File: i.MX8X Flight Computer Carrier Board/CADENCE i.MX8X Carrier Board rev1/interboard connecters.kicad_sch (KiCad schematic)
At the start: 54 parts, among them CN2 DF11-16DP-2DSA(08), CN3 DF11-16DP-2DSA(08), CN4 DF11-16DP-2DSA(08), J10 Conn_01x04, J11 Conn_01x04, J13 Conn_01x04, J16 Conn_01x04, J17 Conn_01x04, J21 Conn_02x02_Odd_Even, J22 Conn_01x04, J23 Conn_01x04, J24 Conn_01x05, J25 Conn_01x05, J27 Conn_01x04, J6 Conn_01x01, J7 Conn_01x08, J8 Conn_02x26_Odd_Even, J9 Conn_02x26_Odd_Even, U33 SN65HVD233, U34 INA219AxDCN, U35 TPS22810DBV, U36 INA219AxDCN, U37 TPS22810DBV, U38 INA219AxDCN, U39 TPS22975

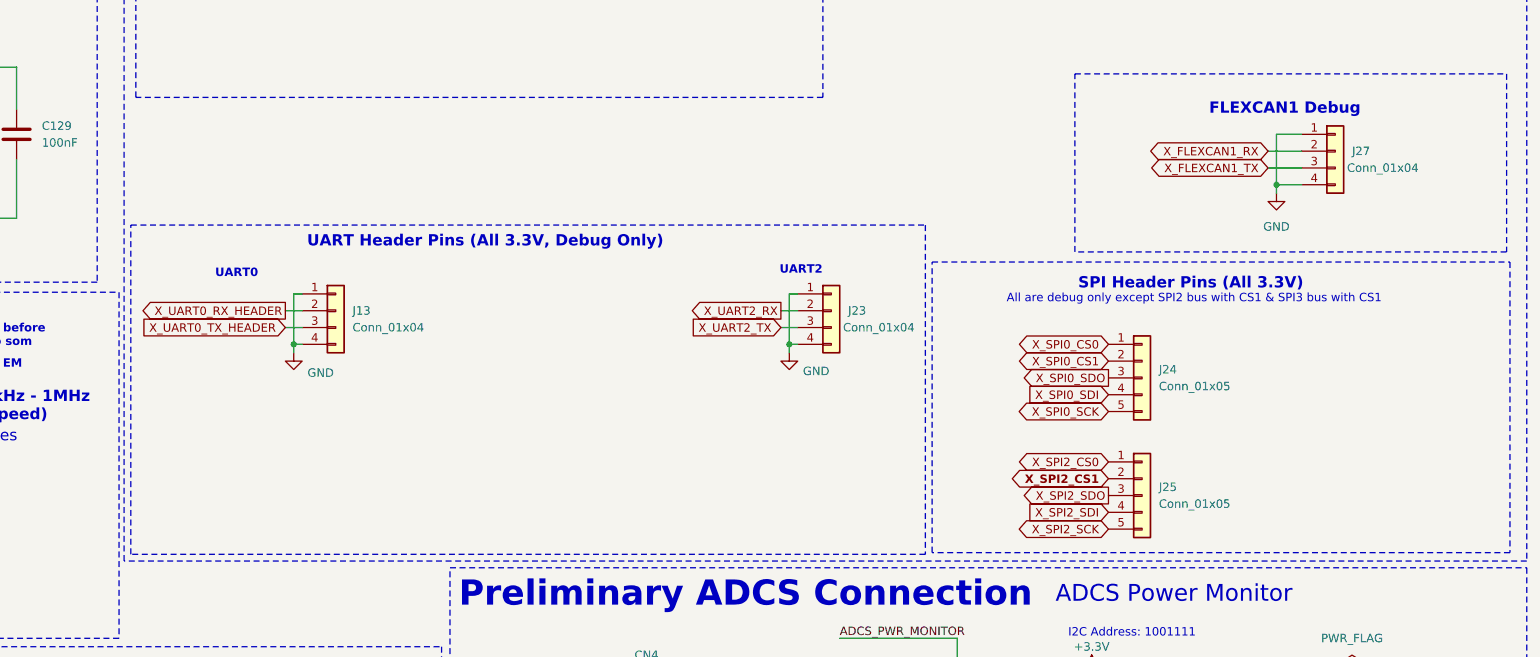
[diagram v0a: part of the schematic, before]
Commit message: DRC fixes
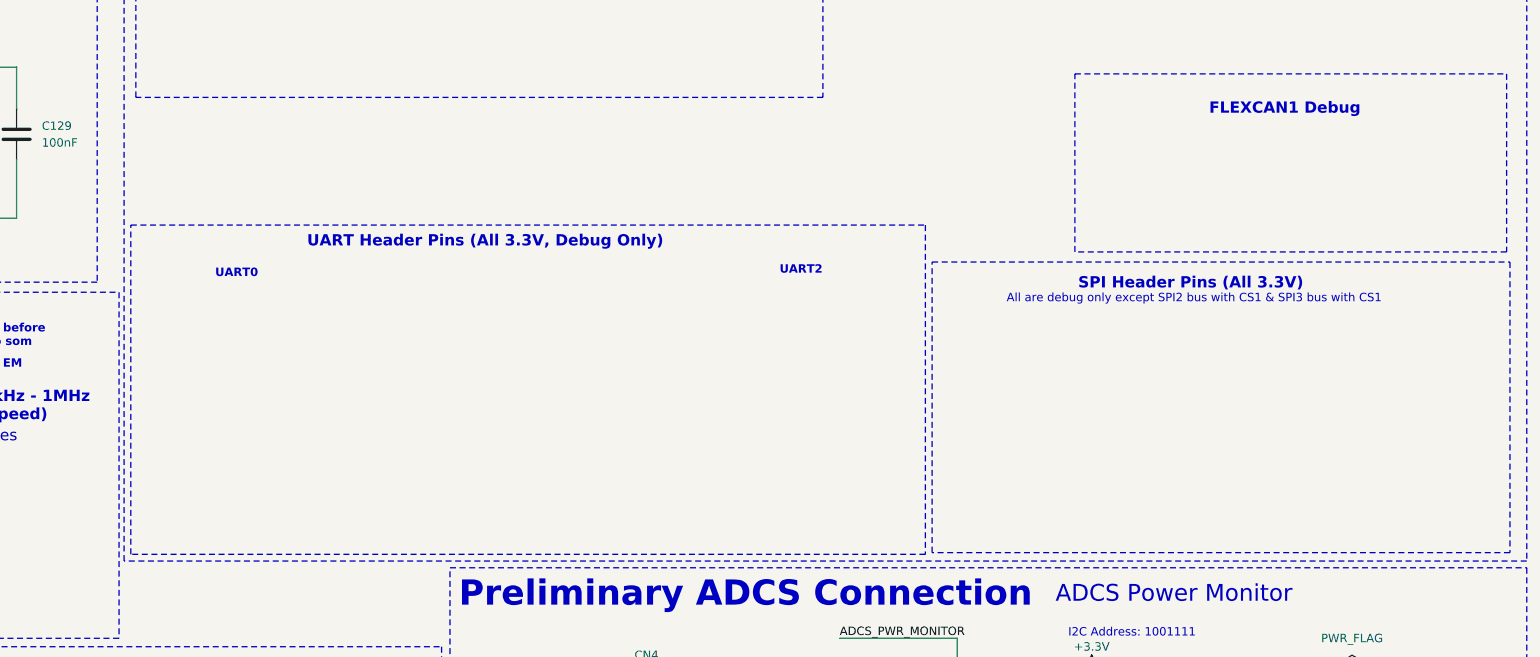
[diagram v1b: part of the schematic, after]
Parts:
- removed J13, J23, J27: Conn_01x04, Connector_PinHeader_1.27mm:PinHeader_1x04_P1.27mm_Vertical, symbol Connector_Generic:Conn_01x04
- removed J24, J25: Conn_01x05, Connector_PinHeader_1.27mm:PinHeader_1x05_P1.27mm_Vertical, symbol Connector_Generic:Conn_01x05
